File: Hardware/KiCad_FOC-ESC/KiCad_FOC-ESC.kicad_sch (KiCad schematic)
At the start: 11 parts, among them U1 STM32G473RCTx

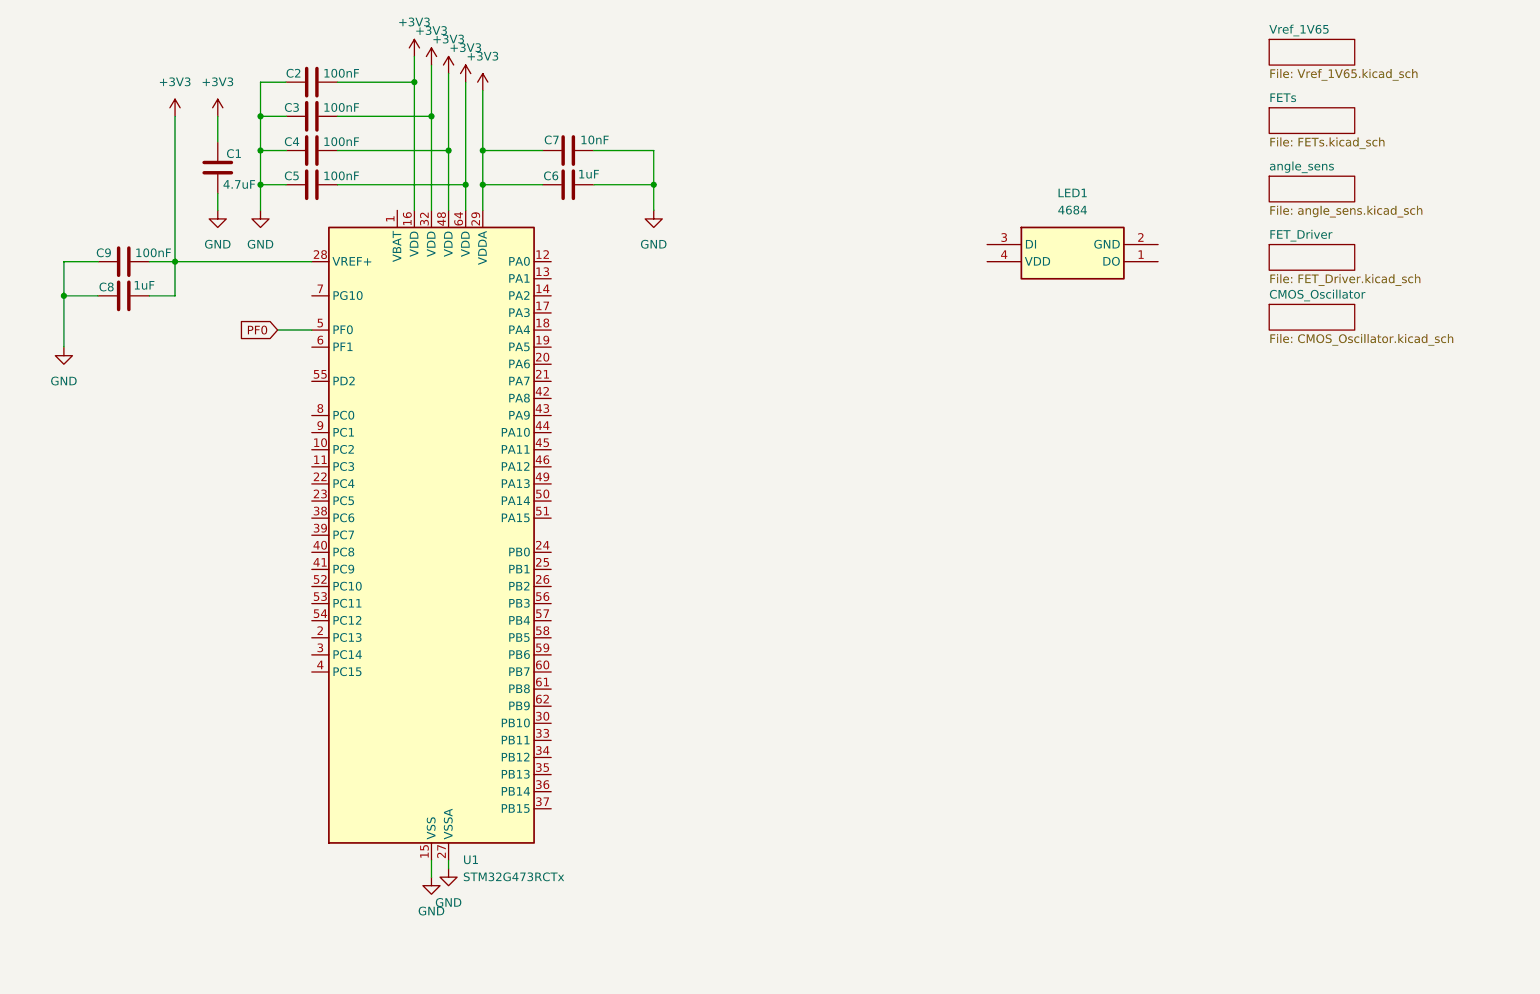
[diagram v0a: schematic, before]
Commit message: initial connections
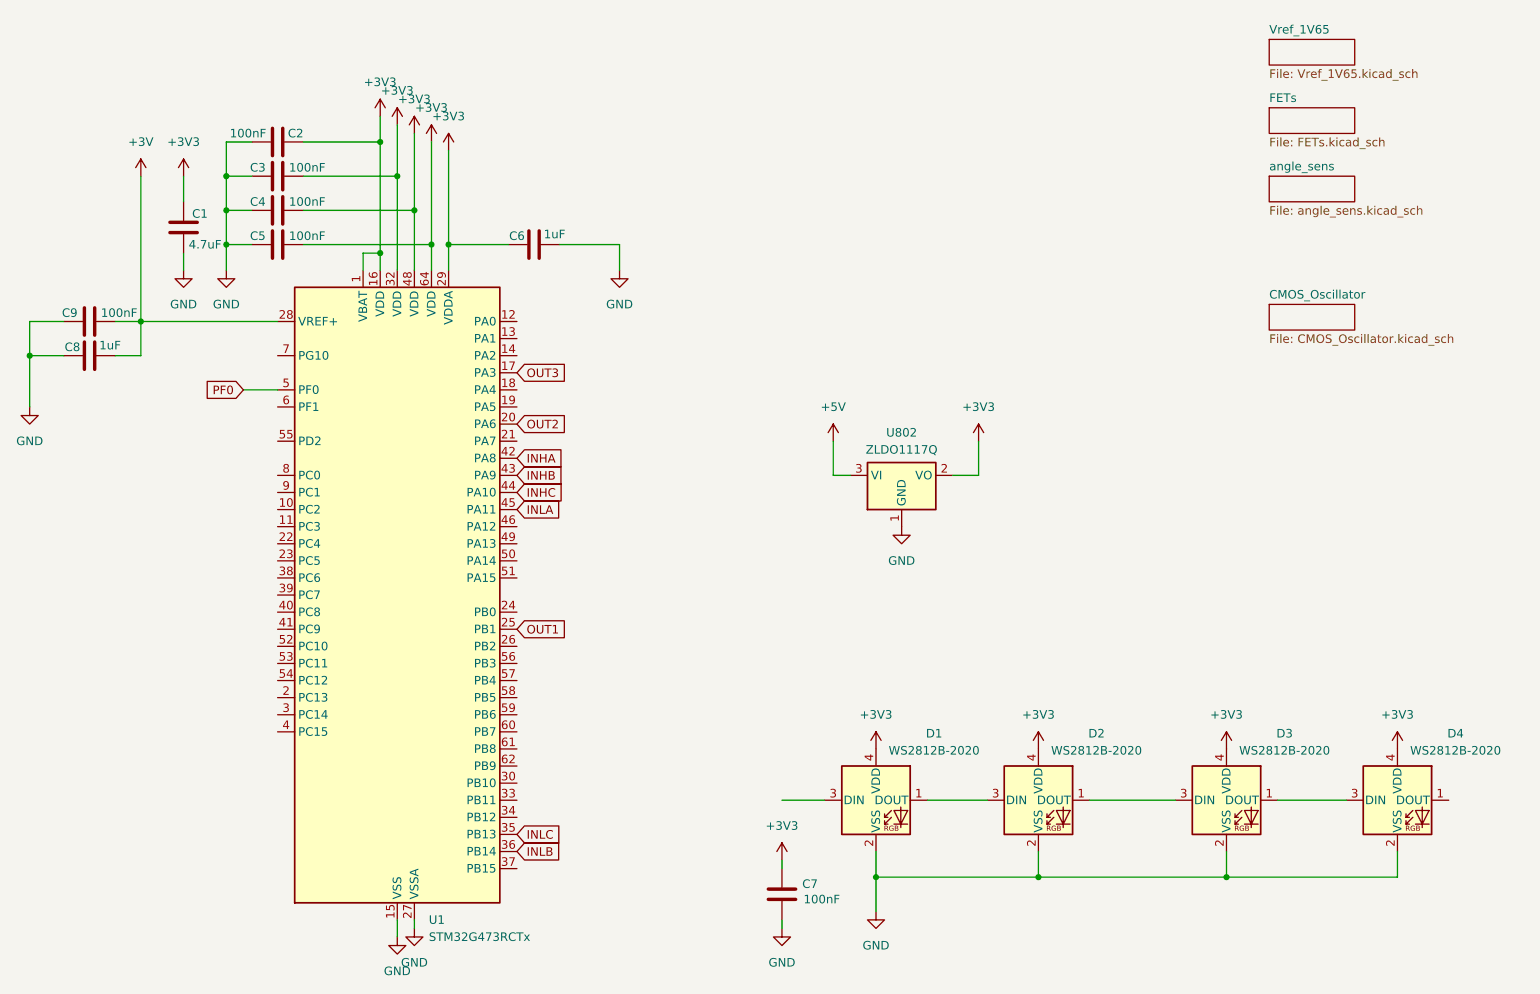
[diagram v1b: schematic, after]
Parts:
- removed LED1: 4684, 4684, symbol SamacSys_Parts1:4684
- added D1, D2, D3, D4: WS2812B-2020, LED_SMD:LED_WS2812B-2020_PLCC4_2.0x2.0mm, symbol LED:WS2812B-2020
- added U802: ZLDO1117Q, Package_TO_SOT_SMD:SOT-223-3_TabPin2, symbol Regulator_Linear:LD1117S33TR_SOT223
- C7: value 10nF -> 100nF
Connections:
- net +3V3: now also C2.1, U1.1 (VBAT), D1.4 (VDD), D2.4 (VDD), D3.4 (VDD), D4.4 (VDD), U802.2 (VO); no longer C2.2, C8.2, C9.2, U1.28 (VREF+)
- net GND: now also C2.2, D1.2 (VSS), D2.2 (VSS), D3.2 (VSS), D4.2 (VSS), U802.1 (GND); no longer C2.1
- net OUT3: now reaches U1.17 (PA3)
- net OUT2: now reaches U1.20 (PA6)
- net OUT1: now reaches U1.25 (PB1)
- net INLC: now reaches U1.35 (PB13)
- net INLB: now reaches U1.36 (PB14)
- net INHA: now reaches U1.42 (PA8)
- net INHB: now reaches U1.43 (PA9)
- net INHC: now reaches U1.44 (PA10)
- net INLA: now reaches U1.45 (PA11)
- new net: D2.1 (DOUT), D3.3 (DIN)
- new net: D1.1 (DOUT), D2.3 (DIN)
- new net: D3.1 (DOUT), D4.3 (DIN)
- new net +3V: C8.2, C9.2, U1.28 (VREF+)
- new net +5V: U802.3 (VI)
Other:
- removed sheet FET_Driver
- moved on the sheet: C1, C2, C3, C4, C5, C6, C8, C9, U1
